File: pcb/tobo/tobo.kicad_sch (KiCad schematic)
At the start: 99 parts, among them J1 54548-2272, J2 Conn_01x02_Pin, J4 54548-2472, J5 Conn_01x09_Pin, J6 Conn_01x09_Pin, J7 Conn_01x09_Pin, J8 Hroparts Elec TYPE-C-31-M-12, U1 TS5A23167DCUR, U10 5015, U11 5015, U12 5015, U13 5015, U14 CH340E, U15 5015, U16 5015, U17 TLV61220ADBVR, U18 MAXM20343AMP+, U2 ATmega328P-AN, U3 TS5A23167DCUR, U4 TS5A23167DCUR, U5 TS5A23167DCUR, U6 5015, U7 5015, U8 5015, U9 5015, X1 TestPoint, X2 TestPoint, X7 TestPoint, Y4 TestPoint

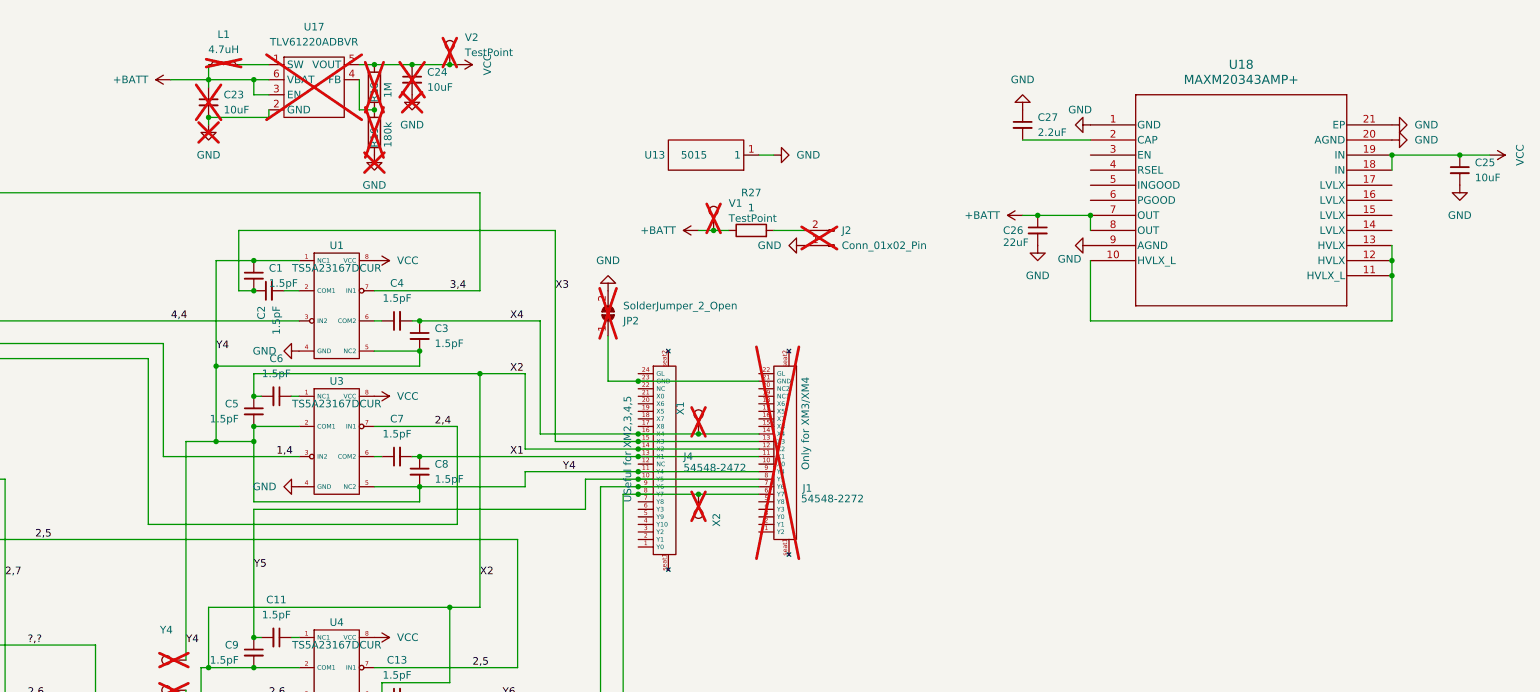
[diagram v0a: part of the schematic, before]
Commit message: Minor versioning shenanigans
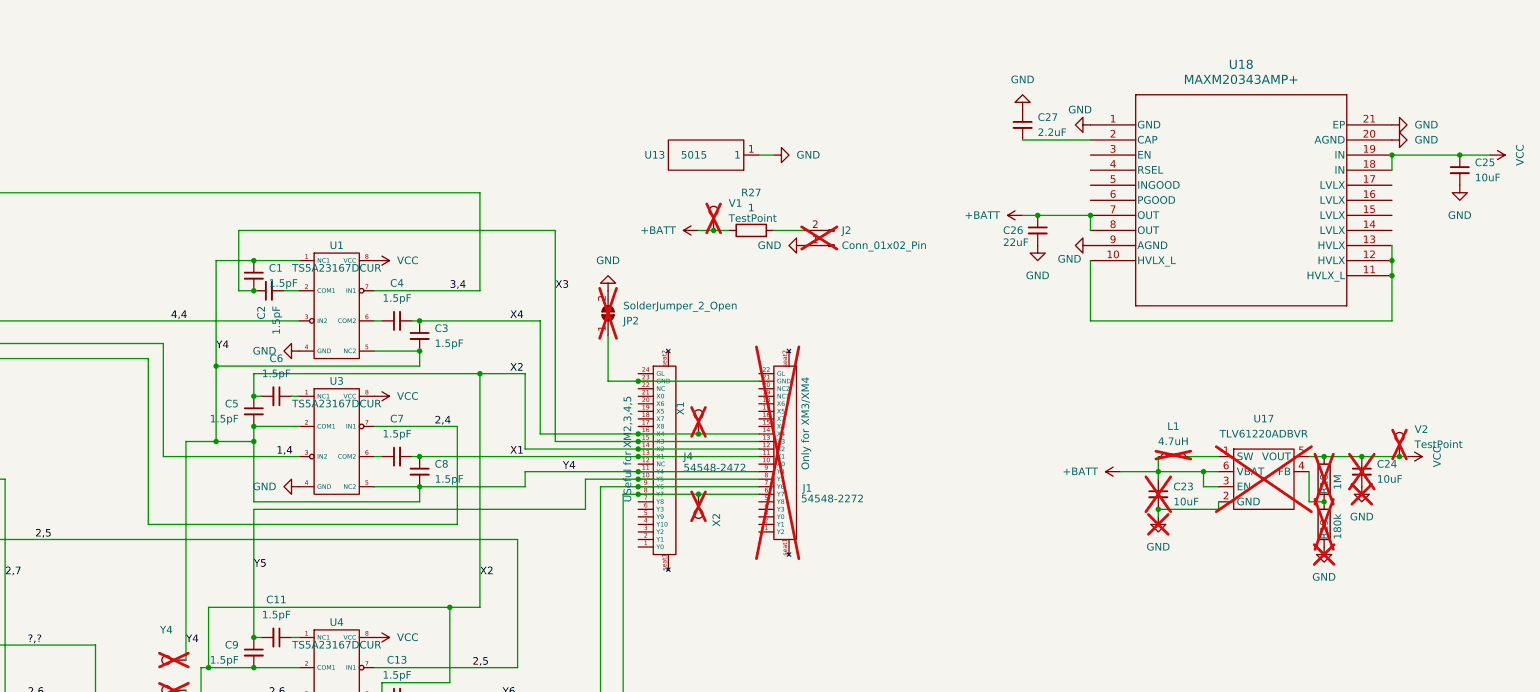
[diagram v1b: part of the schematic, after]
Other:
- moved on the sheet: C23, C24, L1, R18, R19, U17, V2
